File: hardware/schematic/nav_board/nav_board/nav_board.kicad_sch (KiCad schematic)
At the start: 7 parts, among them J1 Conn_01x04_Pin, SW1 SW_Push, SW2 SW_Push

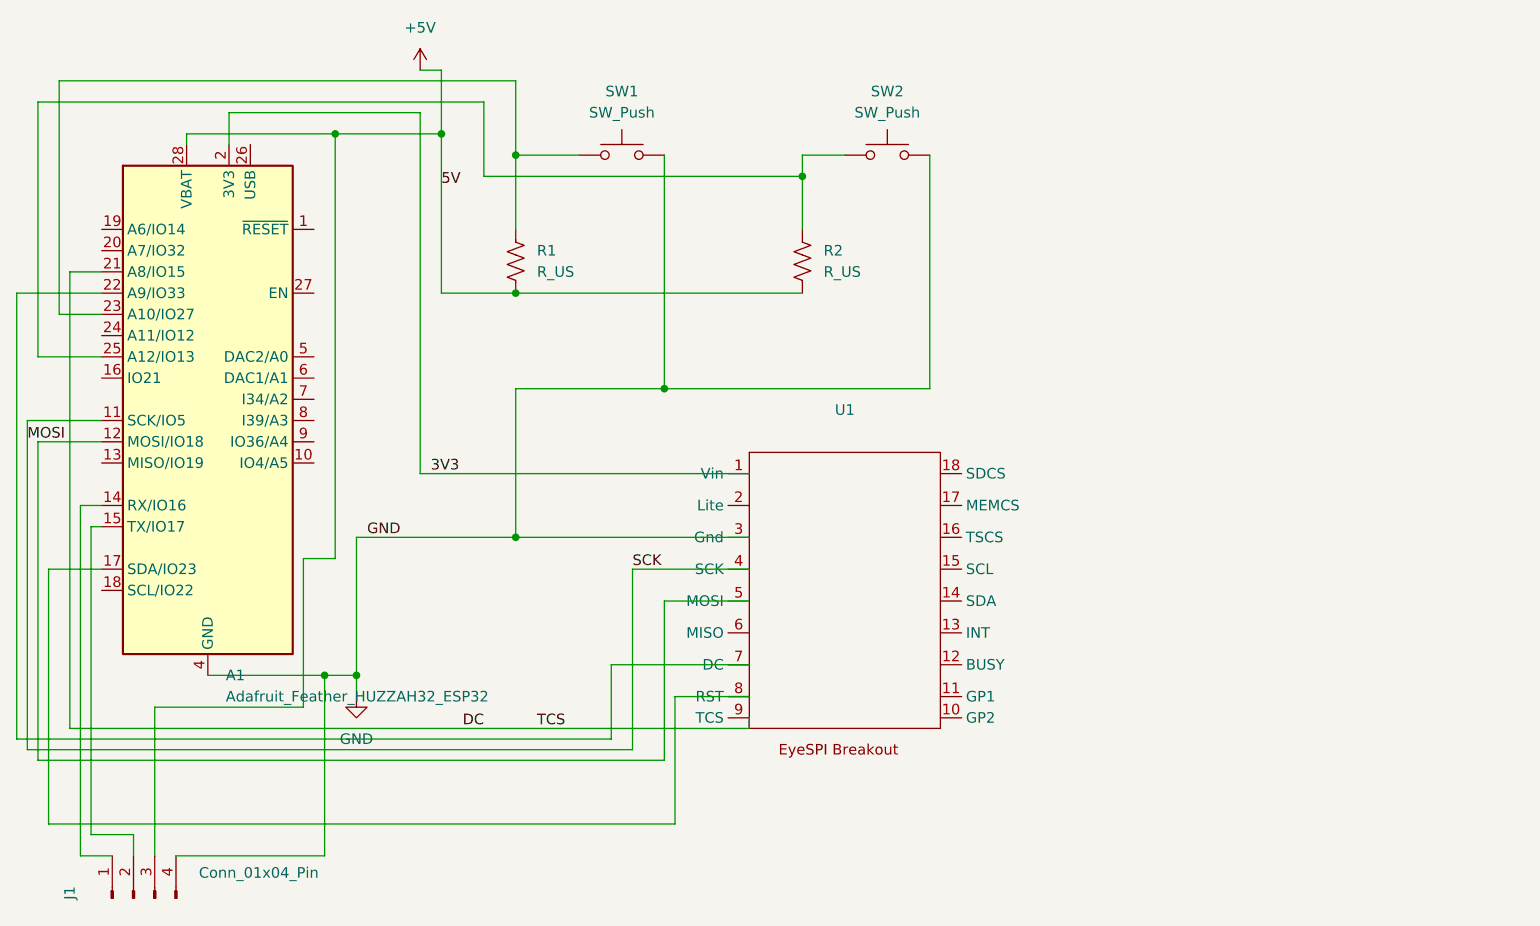
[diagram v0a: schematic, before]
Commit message: First version of Nav PCB
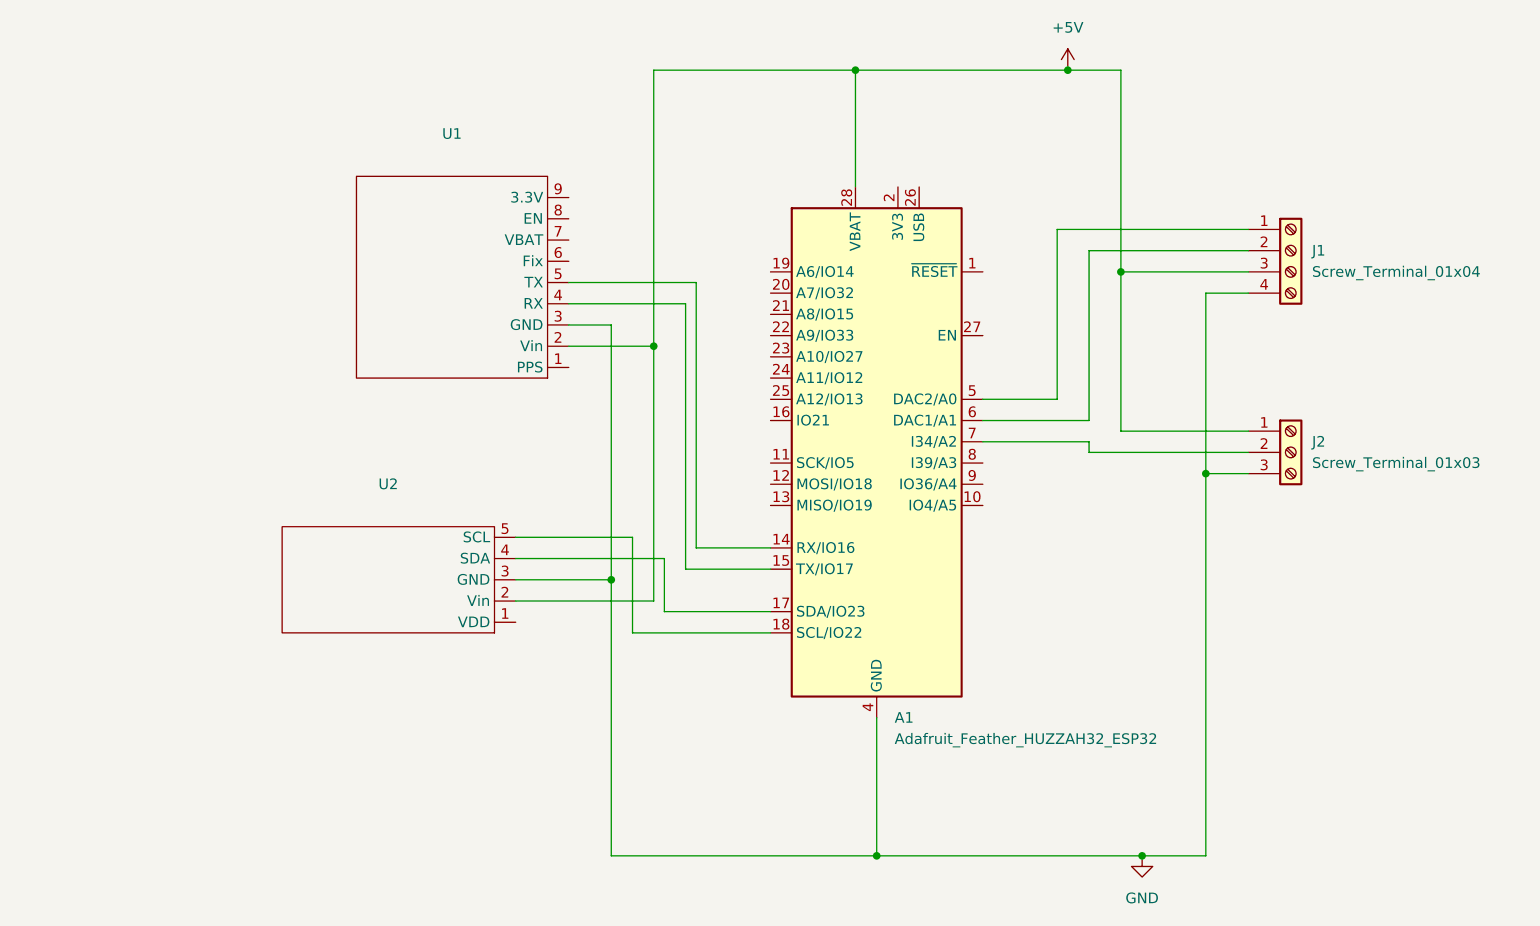
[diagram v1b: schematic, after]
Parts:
- removed J1: Conn_01x04_Pin, TerminalBlock:TerminalBlock_MaiXu_MX126-5.0-04P_1x04_P5.00mm, symbol Connector:Conn_01x04_Pin
- removed R1, R2: R_US, Resistor_THT:R_Axial_DIN0207_L6.3mm_D2.5mm_P7.62mm_Horizontal, symbol Device:R_US
- removed SW1, SW2: SW_Push, TerminalBlock:TerminalBlock_MaiXu_MX126-5.0-02P_1x02_P5.00mm, symbol Switch:SW_Push
- removed U1: ~, DPV_Nav_Library:EyeSPI_Breakout, symbol New_Library:EyeSpi_Breakout
- added J1: Screw_Terminal_01x04, TerminalBlock:TerminalBlock_MaiXu_MX126-5.0-04P_1x04_P5.00mm, symbol Connector:Screw_Terminal_01x04
- added J2: Screw_Terminal_01x03, TerminalBlock:TerminalBlock_MaiXu_MX126-5.0-03P_1x03_P5.00mm, symbol Connector:Screw_Terminal_01x03
- added U1: ~, DPVNav Footprint Library:Adafruit Ultimate GPS, symbol MCU_Module:Adafruit_Ultimate_GPS
- added U2: ~, DPVNav Footprint Library:Pololu Altimu-10 v5, symbol MCU_Module:Pololu_Altimu-10_v5
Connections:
- net +5V: now also J1.3 (Pin_3), J2.1 (Pin_1), U1.2 (Vin), U2.2 (Vin)
- net GND: now also J1.4 (Pin_4), J2.3 (Pin_3), U1.3 (GND), U2.3 (GND)
- net at A1.14 (RX/IO16): now also U1.5 (TX)
- net at A1.15 (TX/IO17): now also U1.4 (RX)
- net at A1.17 (SDA/IO23): now also U2.4 (SDA)
- net at A1.18 (SCL/IO22): now also U2.5 (SCL)
- net at A1.5 (DAC2/A0): now also J1.1 (Pin_1)
- net at A1.6 (DAC1/A1): now also J1.2 (Pin_2)
- net at A1.7 (I34/A2): now also J2.2 (Pin_2)
- net 3V3: no longer names the net of A1.2 (3V3)
- net DC: no longer names the net of A1.21 (A8/IO15)
- net MOSI: no longer names the net of A1.11 (SCK/IO5)
